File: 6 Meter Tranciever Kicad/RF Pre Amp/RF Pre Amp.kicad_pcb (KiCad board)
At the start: 2 copper layers, 52 parts, among them J1 RF In, J2 RF Out, J3 Conn_01x03_Male, J4 Conn_01x03_Male, Q1 BFR106, Q10 BFR106, Q2 BFR106, Q3 AO3400A, Q4 AO3401A, Q5 BFR106, Q6 BFR106, Q7 BFR106, Q8 BFR106, Q9 BFR106, T1 T43-37 Trifillar 10 Turns, T2 T43-37 Trifillar 10 Turns

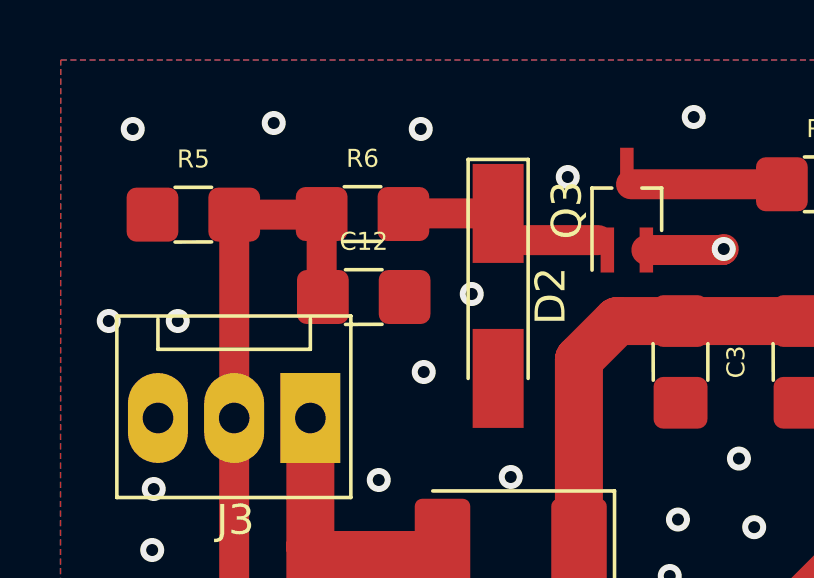
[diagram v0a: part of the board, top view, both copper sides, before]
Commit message: Board tweaks
Board tweaks and remove bak files
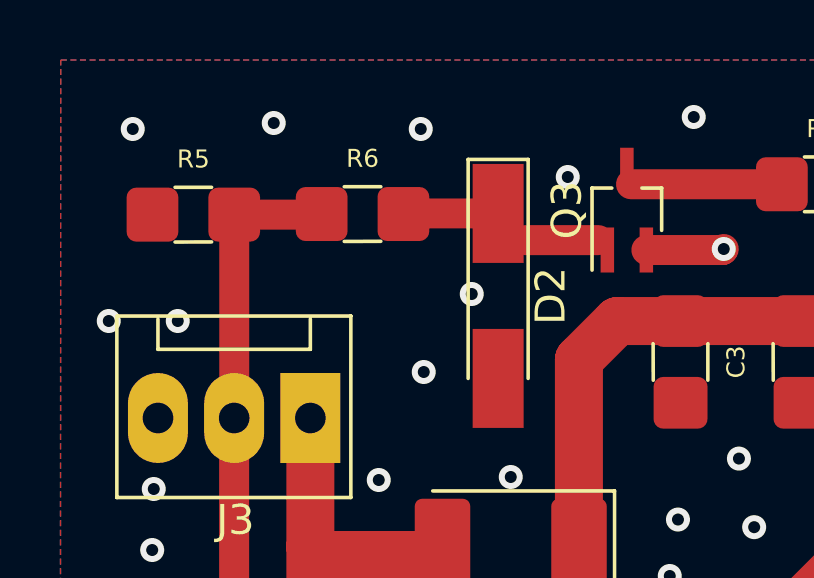
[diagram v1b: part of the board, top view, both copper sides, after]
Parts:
- removed C12: 33n, WC8C:SMD_Combo_1206_0805
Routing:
- net /RX_Low_TX_High: track 22.5 -> 19.8 mm
